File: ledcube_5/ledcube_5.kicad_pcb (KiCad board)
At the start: 2 copper layers, 104.1 x 89.9 mm, 74 parts, among them J1 Conn_01x05_MountingPin, J2 Conn_01x01, J3 Conn_01x01, J4 Conn_01x01, J5 Conn_01x01, J6 Conn_01x01, Q1 PN2222A, Q2 PN2222A, Q3 PN2222A, Q4 PN2222A, Q5 PN2222A, U1 74HC595, U2 74HC595, U3 74HC595, U4 74HC595

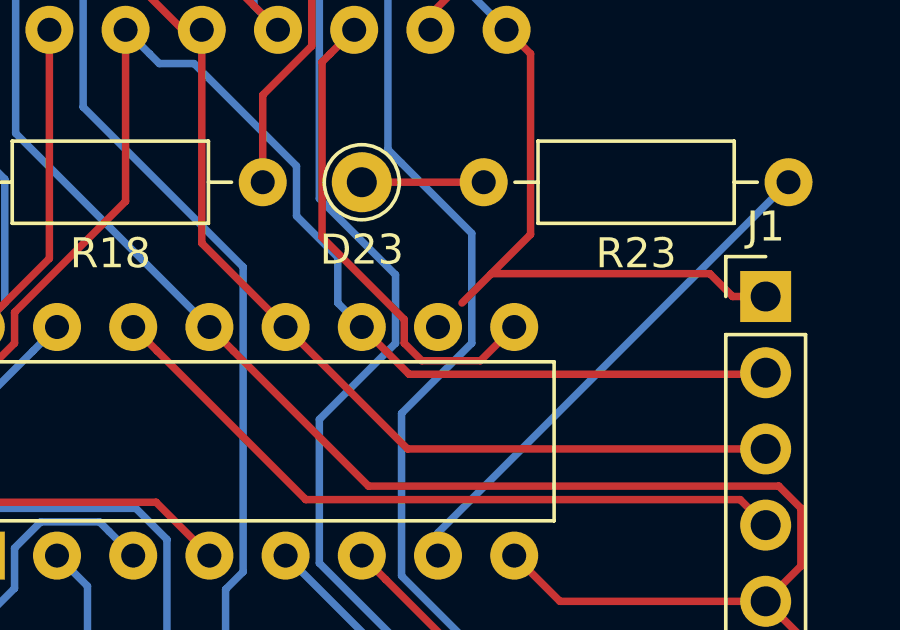
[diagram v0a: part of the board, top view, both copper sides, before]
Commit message: why
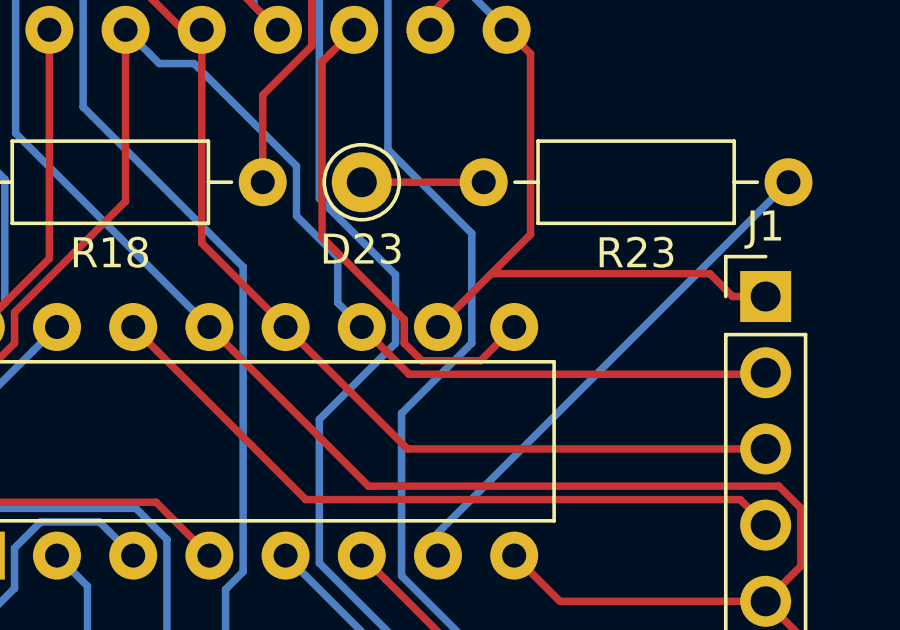
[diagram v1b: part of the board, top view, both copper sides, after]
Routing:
- net +5V: track 210.6 -> 211.7 mm
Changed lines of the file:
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@@
     (thickness 1.6)
     (drawings 10)
-    (tracks 454)
+    (tracks 455)
     (zones 0)
     (modules 74)
@@
       (outputformat 1)
       (mirror false)
-      (drillshape 1)
+      (drillshape 0)
       (scaleselection 1)
       (outputdirectory ""))
@@
   (segment (start 246.804 81.28) (end 239.522 81.28) (width 0.25) (layer F.Cu) (net 30))
   (segment (start 240.829999 79.972001) (end 239.522 81.28) (width 0.25) (layer F.Cu) (net 30))
+  (segment (start 237.744 83.058) (end 238.543999 82.258001) (width 0.25) (layer F.Cu) (net 30))
   (segment (start 224.244001 83.857999) (end 225.044 83.058) (width 0.25) (layer B.Cu) (net 31))
   (segment (start 215.501001 92.600999) (end 224.244001 83.857999) (width 0.25) (layer B.Cu) (net 31))
@@
   (segment (start 227.673991 89.102989) (end 223.029011 89.102989) (width 0.25) (layer B.Cu) (net 32))
   (segment (start 228.709001 90.137999) (end 227.673991 89.102989) (width 0.25) (layer B.Cu) (net 32))
-  (segment (start 233.426 104.394) (end 233.68 104.14) (width 0.25) (layer F.Cu) (net 72))
   (segment (start 226.06 91.694) (end 225.044 90.678) (width 0.25) (layer B.Cu) (net 33))
   (segment (start 226.06 99.06) (end 226.06 91.694) (width 0.25) (layer B.Cu) (net 33))
@@
   (segment (start 213.36 99.06) (end 214.886989 97.533011) (width 0.25) (layer B.Cu) (net 34))
   (segment (start 211.385997 97.083001) (end 219.568998 88.9) (width 0.25) (layer F.Cu) (net 35))
-  (segment (start 192.532 104.394) (end 192.532 103.394) (width 0.25) (layer F.Cu) (net 76))
   (segment (start 228.346 88.9) (end 230.124 90.678) (width 0.25) (layer F.Cu) (net 35))
   (segment (start 219.568998 88.9) (end 228.346 88.9) (width 0.25) (layer F.Cu) (net 35))
@@
   (segment (start 247.62499 101.09499) (end 196.10101 101.09499) (width 0.25) (layer F.Cu) (net 71))
   (segment (start 249.4 102.87) (end 247.62499 101.09499) (width 0.25) (layer F.Cu) (net 71))
+  (segment (start 233.426 104.394) (end 233.68 104.14) (width 0.25) (layer F.Cu) (net 72))
   (segment (start 233.426 104.394) (end 233.68 104.14) (width 0.25) (layer B.Cu) (net 72))
   (segment (start 233.426 105.394) (end 233.426 104.394) (width 0.25) (layer B.Cu) (net 72))
@@
   (segment (start 202.692 99.568) (end 203.2 99.06) (width 0.25) (layer B.Cu) (net 75))
   (segment (start 202.692 104.394) (end 202.692 99.568) (width 0.25) (layer B.Cu) (net 75))
+  (segment (start 192.532 104.394) (end 192.532 103.394) (width 0.25) (layer F.Cu) (net 76))
   (segment (start 192.532 101.092) (end 190.5 99.06) (width 0.25) (layer F.Cu) (net 76))
   (segment (start 192.532 104.394) (end 192.532 101.092) (width 0.25) (layer F.Cu) (net 76))
